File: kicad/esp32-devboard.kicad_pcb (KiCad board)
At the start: 4 copper layers, 76 x 54.5 mm, 21 parts, among them J1 Conn_01x20, J2 Conn_01x20, J3 USB_C_Receptacle_USB2.0_16P, SW1 SW_Push, SW2 SW_Push, U1 ESP32-S3-WROOM-1, U2 LD1117S33TR_SOT223

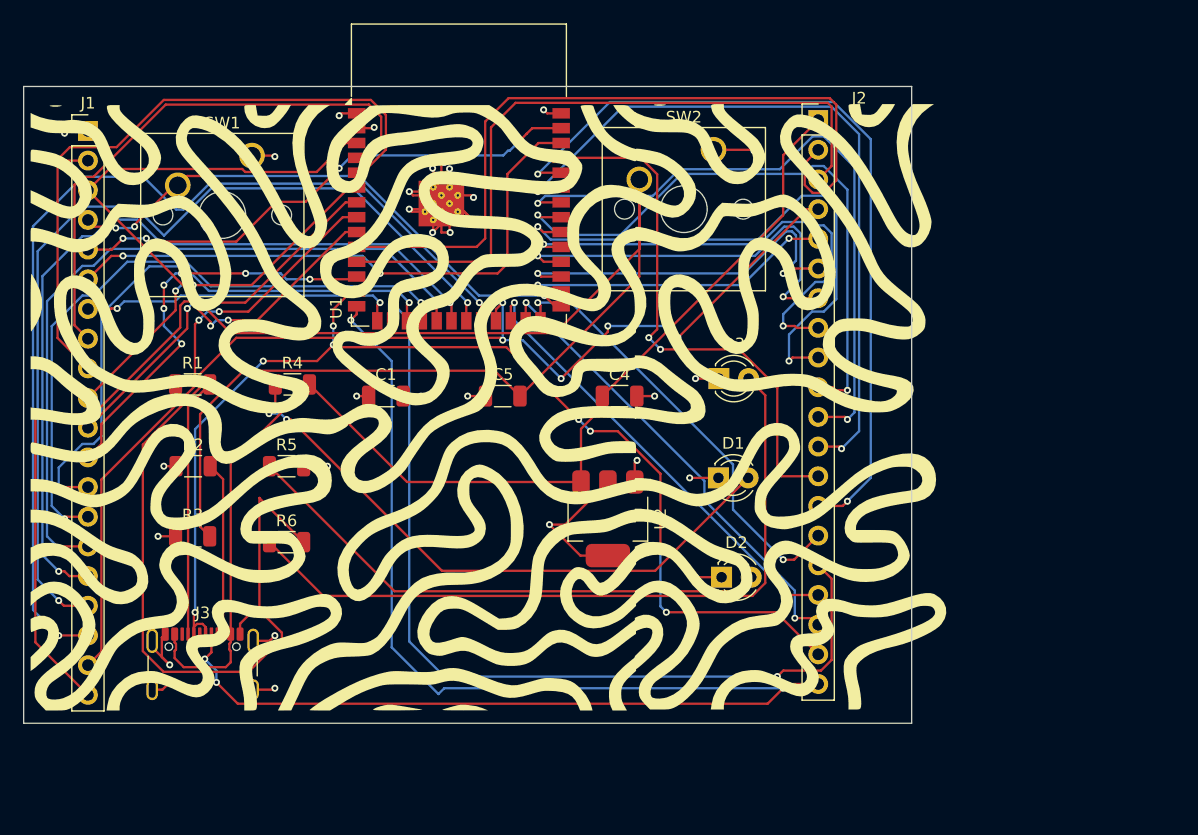
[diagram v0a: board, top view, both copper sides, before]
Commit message: added
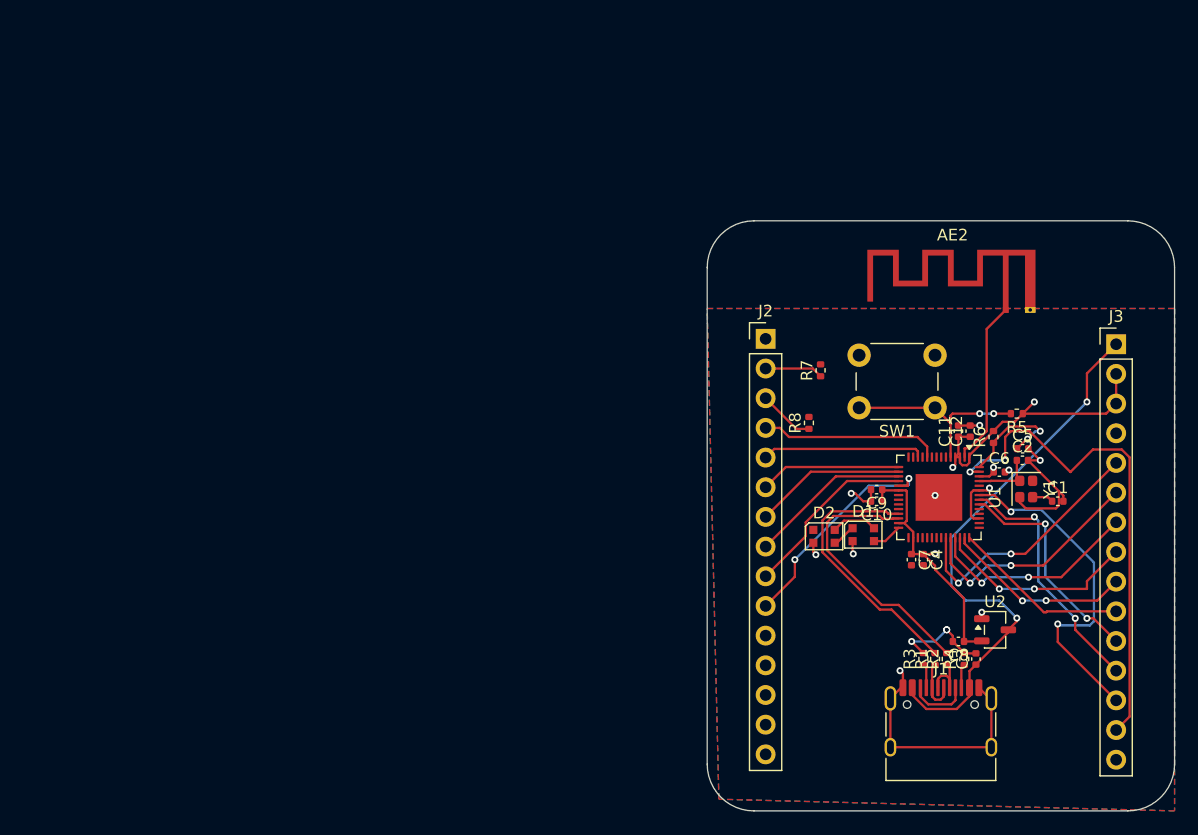
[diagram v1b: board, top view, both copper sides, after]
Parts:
- removed D3: LED, LED_THT:LED_D3.0mm
- removed G*** (x2): LOGO, LOGO
- removed SW2: SW_Push, Button_Switch_Keyboard:SW_Cherry_MX_1.00u_PCB
- added AE2: Antenna_Shield, RF_Antenna:Texas_SWRA117D_2.4GHz_Left, F.Cu at (191.1, 89.6)
- added C10: 1uF, Capacitor_SMD:C_0402_1005Metric, F.Cu at (180.0, 106.0)
- added C11: 1uF, Capacitor_SMD:C_0402_1005Metric, F.Cu at (187.0, 100.0)
- added C12: 100nF, Capacitor_SMD:C_0402_1005Metric, F.Cu at (188.0, 100.0)
- added C2: 33pF, Capacitor_SMD:C_0402_1005Metric, F.Cu at (192.5, 102.5)
- added C3: 4.7uf, Capacitor_SMD:C_0402_1005Metric, F.Cu at (188.5, 119.5)
- added C6: 1uF, Capacitor_SMD:C_0402_1005Metric, F.Cu at (190.5, 103.5)
- added C7: 1uF, Capacitor_SMD:C_0402_1005Metric, F.Cu at (183.0, 111.0)
- added C8: 1uF, Capacitor_SMD:C_0402_1005Metric, F.Cu at (187.0, 118.0)
- added C9: 1uF, Capacitor_SMD:C_0402_1005Metric, F.Cu at (180.0, 105.0)
- added R7: 10K, Resistor_SMD:R_0402_1005Metric, F.Cu at (175.2, 94.8)
- added R8: 10K, Resistor_SMD:R_0402_1005Metric, F.Cu at (174.2, 99.3)
- added Y1: 25MHz 20pF, Crystal:Crystal_SMD_2016-4Pin_2.0x1.6mm, F.Cu at (192.8, 105.0)
- C1: value 10uF -> 33pF; footprint Capacitor_SMD:C_1206_3216Metric -> Capacitor_SMD:C_0402_1005Metric
- C4: value 100nF -> 4.7uf; footprint Capacitor_SMD:C_1206_3216Metric -> Capacitor_SMD:C_0402_1005Metric
- C5: value 10uF -> 1uF; footprint Capacitor_SMD:C_1206_3216Metric -> Capacitor_SMD:C_0402_1005Metric
- D1, D2: value LED -> WS2812B-2020; footprint LED_THT:LED_D3.0mm -> LED_SMD:LED_WS2812B-2020_PLCC4_2.0x2.0mm
- J1: value Conn_01x20 -> USB_C_Receptacle_USB2.0_14P; footprint Connector_PinHeader_2.54mm:PinHeader_1x20_P2.54mm_Vertical -> Connector_USB:USB_C_Receptacle_HRO_TYPE-C-31-M-12
- J2: value Conn_01x20 -> Conn_01x15; footprint Connector_PinHeader_2.54mm:PinHeader_1x20_P2.54mm_Vertical -> Connector_PinHeader_2.54mm:PinHeader_1x15_P2.54mm_Vertical
- J3: value USB_C_Receptacle_USB2.0_16P -> Conn_01x15; footprint Connector_USB:USB_C_Receptacle_GCT_USB4105-xx-A_16P_TopMnt_Horizontal -> Connector_PinHeader_2.54mm:PinHeader_1x15_P2.54mm_Vertical
- R1, R2, R4, R5: footprint Resistor_SMD:R_1206_3216Metric -> Resistor_SMD:R_0402_1005Metric
- R3: value 51.k -> 5.1k; footprint Resistor_SMD:R_1206_3216Metric -> Resistor_SMD:R_0402_1005Metric
- R6: value 5.1k -> 10k; footprint Resistor_SMD:R_1206_3216Metric -> Resistor_SMD:R_0402_1005Metric
- SW1: footprint Button_Switch_Keyboard:SW_Cherry_MX_1.00u_PCB -> Button_Switch_THT:SW_PUSH_6mm
- U1: value ESP32-S3-WROOM-1 -> ESP32-S2; footprint RF_Module:ESP32-S3-WROOM-1 -> Package_DFN_QFN:QFN-56-1EP_7x7mm_P0.4mm_EP4x4mm
- U2: value LD1117S33TR_SOT223 -> XC6206PxxxMR; footprint Package_TO_SOT_SMD:SOT-223-3_TabPin2 -> Package_TO_SOT_SMD:SOT-23-3
- moved J1 89.5 mm to (185.5, 126.0)
- moved J3 83.2 mm to (200.5, 92.6)
- moved R1 67.7 mm to (185.0, 119.5), turned to 90 degrees
- moved R2 66.6 mm to (186.0, 119.5), turned to 90 degrees
- moved R3 63.4 mm to (184.0, 119.5), turned to 90 degrees
- moved R5 62.7 mm to (192.0, 98.5), turned to 180 degrees
- moved SW1 62.3 mm to (185.0, 98.0), turned to 180 degrees
- moved R4 62.1 mm to (187.5, 119.5), turned to 90 degrees
- moved R6 61.2 mm to (190.0, 100.5), turned to 90 degrees
- moved C1 58.2 mm to (195.5, 106.0)
- moved U1 49.5 mm to (185.3, 105.7), turned to -90 degrees
- moved C5 44.7 mm to (192.5, 101.5)
- moved U2 34.5 mm to (190.1, 117.0), turned to 0 degrees
- moved C4 29.5 mm to (184.0, 111.0), turned to -90 degrees
- moved J2 19.3 mm to (170.5, 92.1)
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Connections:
- C1 pad 1: +3V3 -> /XO
- C4 pad 1: +5V -> +3V3
- C5 pad 1: GND -> /CHIP_PU
- C5 pad 2: /EN -> GND
- D1 pad 1: GND -> Net-(D1-DOUT)
- D1 pad 2: Net-(D1-A) -> GND
- D2 pad 1: GND -> unconnected-(D2-DOUT-Pad1)
- D2 pad 2: Net-(D2-A) -> GND
- J2 pad 1: +5V -> GND
- J2 pad 10: /GPIO40 -> /GPIO14
- J2 pad 11: /GPIO41 -> /GPIO15
- J2 pad 12: /GPIO42 -> /GPIO16
- J2 pad 13: /GPIO43 / TXD0 -> GND
- J2 pad 14: /GPIO44 / RXD0 -> GND
- J2 pad 15: /GPIO45 -> GND
- J2 pad 2: /GPIO17 -> /SWCLK
- J2 pad 3: /GPIO18 -> /SWDIO
- J2 pad 4: /GPIO21 -> /GPIO5
- J2 pad 5: /GPIO35 -> /GPIO7
- J2 pad 6: /GPIO36 -> /GPIO10
- J2 pad 7: /GPIO37 -> /GPIO11
- J2 pad 8: /GPIO38 -> /GPIO12
- J2 pad 9: /GPIO39 -> /GPIO13
- R1 pad 1: GND -> /D-
- R1 pad 2: Net-(J3-CC1) -> Net-(U1-GPIO19/USB_D-)
- R2 pad 1: GND -> /D+
- R2 pad 2: Net-(J3-CC2) -> Net-(U1-GPIO20/USB_D+)
- R3 pad 1: +3V3 -> Net-(J1-CC1)
- R3 pad 2: /EN -> GND
- R4 pad 1: Net-(D1-A) -> Net-(J1-CC2)
- R4 pad 2: +5V -> GND
- R5 pad 1: Net-(D2-A) -> +3V3
- R5 pad 2: +3V3 -> /IO0
- R6 pad 1: Net-(D3-A) -> /CHIP_PU
- R6 pad 2: /GPIO21 -> +3V3
- SW1 pad 1: GND -> /IO0
- SW1 pad 2: /GPIO0 -> GND
- U1 pad 1: GND -> +3V3
- U1 pad 10: /GPIO17 -> /GPIO5
- U1 pad 11: /GPIO18 -> /GPIO6
- U1 pad 12: /GPIO8 -> /GPIO7
- U1 pad 13: /USB_D- -> /GPIO8
- U1 pad 14: /USB_D+ -> /GPIO9
- U1 pad 15: /GPIO3 -> /GPIO10
- U1 pad 16: /GPIO46 -> /GPIO11
- U1 pad 17: /GPIO9 -> /GPIO12
- U1 pad 18: /GPIO10 -> /GPIO13
- U1 pad 19: /GPIO11 -> /GPIO14
- U1 pad 2: +3V3 -> Net-(AE2-A)
- U1 pad 20: /GPIO12 -> +3V3
- U1 pad 21: /GPIO13 -> unconnected-(U1-XTAL_32K_P-Pad21)
- U1 pad 22: /GPIO14 -> unconnected-(U1-XTAL_32K_N-Pad22)
- U1 pad 23: /GPIO21 -> unconnected-(U1-DAC_1-Pad23)
- U1 pad 24: /GPIO47 -> unconnected-(U1-DAC_2-Pad24)
- U1 pad 25: /GPIO48 -> Net-(U1-GPIO19/USB_D-)
- U1 pad 26: /GPIO45 -> Net-(U1-GPIO20/USB_D+)
- U1 pad 27: /GPIO0 -> +3V3
- U1 pad 28: /GPIO35 -> /GPIO21
- U1 pad 29: /GPIO36 -> unconnected-(U1-SPICS1-Pad29)
- U1 pad 3: /EN -> +3V3
- U1 pad 30: /GPIO37 -> +3V3
- U1 pad 31: /GPIO38 -> unconnected-(U1-SPIHD-Pad31)
- U1 pad 32: /GPIO39 -> unconnected-(U1-SPIWP-Pad32)
- U1 pad 33: /GPIO40 -> unconnected-(U1-SPICS0-Pad33)
- U1 pad 34: /GPIO41 -> unconnected-(U1-SPICLK-Pad34)
- U1 pad 35: /GPIO42 -> unconnected-(U1-SPIQ-Pad35)
- U1 pad 36: /GPIO44 / RXD0 -> unconnected-(U1-SPID-Pad36)
- U1 pad 37: /GPIO43 / TXD0 -> /GPIO33
- U1 pad 38: /GPIO2 -> /GPIO34
- U1 pad 39: /GPIO1 -> /GPIO35
- U1 pad 4: /GPIO4 -> +3V3
- U1 pad 40: GND -> /GPIO36
- U1 pad 41: GND -> /GPIO37
- U1 pad 5: /GPIO5 -> /IO0
- U1 pad 6: /GPIO6 -> /GPIO1
- U1 pad 7: /GPIO7 -> /GPIO2
- U1 pad 8: /GPIO15 -> /GPIO3
- U1 pad 9: /GPIO16 -> /GPIO4
- U2 pad 3: +5V -> VBUS
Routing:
- net /EN: track 149.5 -> 0.00 mm
- net /USB_D+: track 126.4 -> 0.00 mm, vias 4 -> 0
- net /GPIO21: track 125.5 -> 2.58 mm, vias 5 -> 0
- net /USB_D-: track 99.6 -> 0.00 mm, vias 10 -> 0
- net +5V: track 100.2 -> 3.95 mm
- net /GPIO44 / RXD0: track 68.9 -> 0.00 mm, vias 2 -> 0
- net /GPIO14: track 86.3 -> 19.4 mm
- net /GPIO17: track 65.8 -> 0.00 mm
- net /GPIO13: track 80.1 -> 15.4 mm, vias 2 -> 0
- net /GPIO42: track 63.2 -> 0.00 mm, vias 2 -> 0
- net /GPIO16: track 63.0 -> 0.00 mm, vias 2 -> 0
- net Net-(D3-A): track 62.9 -> 0.00 mm
- net /GPIO18: track 59.9 -> 0.00 mm
- net /GPIO41: track 57.0 -> 0.00 mm, vias 2 -> 0
- net /GPIO12: track 70.0 -> 13.9 mm, vias 2 -> 0
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- added copper zone on B.Cu, net GND
- added copper zone on F.Cu, net GND
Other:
- board size 76 x 54.5 mm -> 40 x 50.5 mm
